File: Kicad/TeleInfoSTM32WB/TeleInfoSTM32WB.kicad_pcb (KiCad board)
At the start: 2 copper layers, 30 x 48.6 mm, 34 parts, among them J1 Conn_01x02_Female, J2 Conn_01x05_Female, J3 RSP-122811-01, J4 Conn_01x05_Female, SW1 SW_Push, U1 STM32WB55CCUx, U2 SFH620A-1, U3 LM2937xMP, Y1 32.768 KHz, Y2 Crystal_GND24

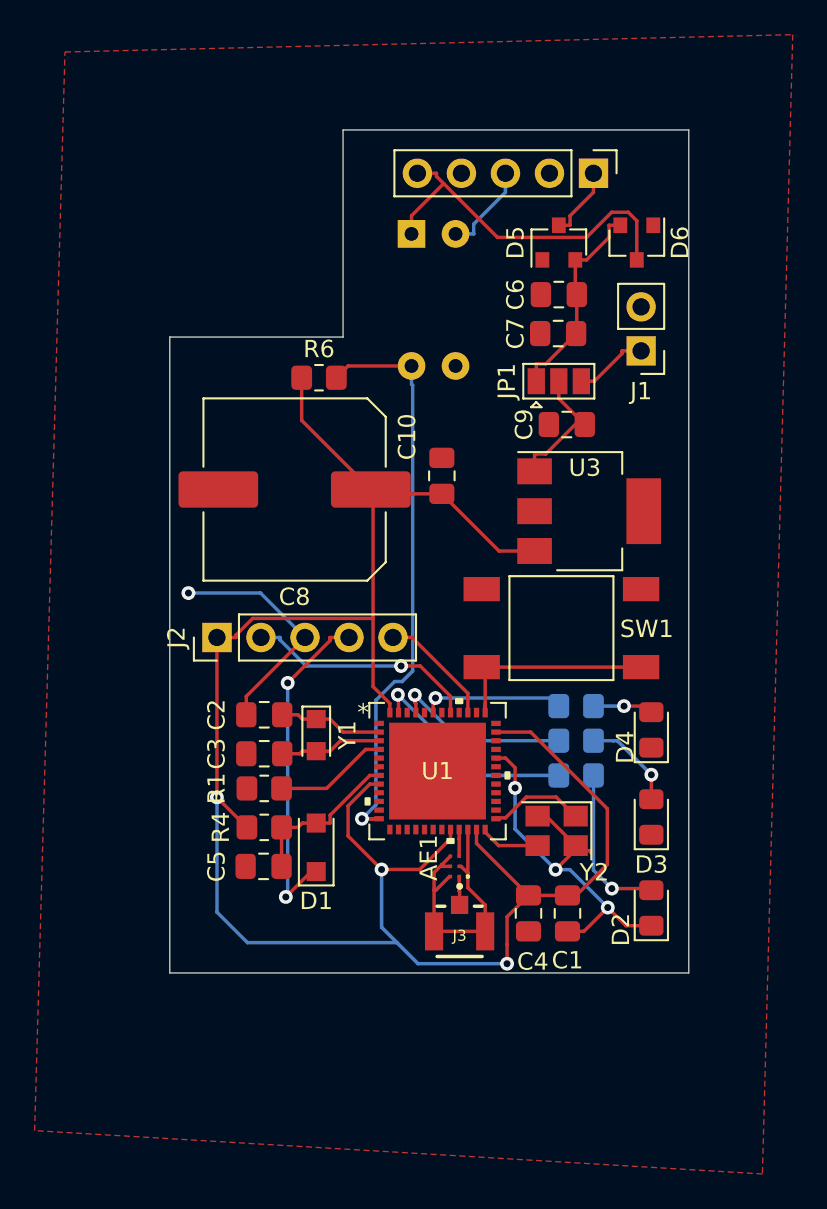
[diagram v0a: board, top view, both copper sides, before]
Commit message: PCB V6 (forget commited filed.... :clap:)
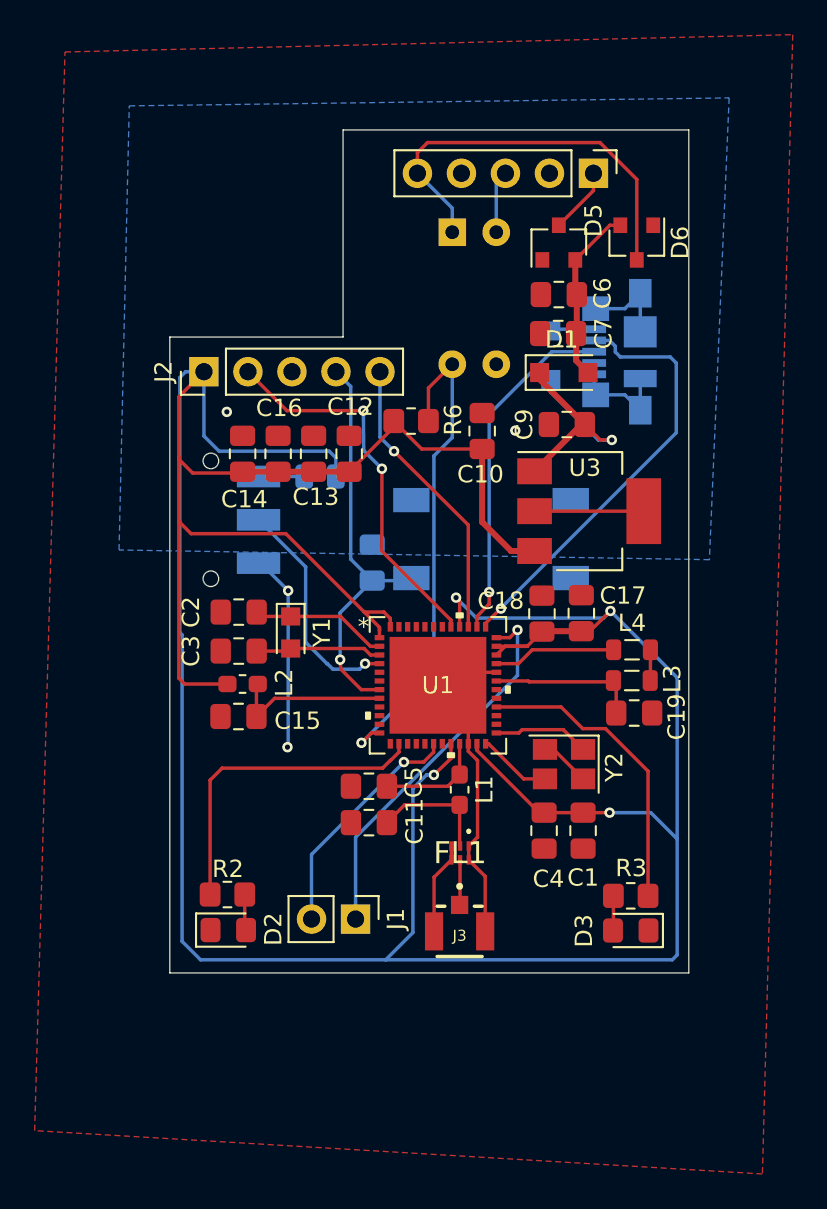
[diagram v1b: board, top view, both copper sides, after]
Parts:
- removed AE1: MLPF-WB55-01E3, MLPF-WB55-01E3:MLPF-WB55-01E3
- removed C8: 470mF, Capacitor_SMD:C_Elec_10x10.2
- removed JP1: Jumper_3_Open, Jumper:SolderJumper-3_P1.3mm_Open_Pad1.0x1.5mm
- removed R1: 10K, Resistor_SMD:R_0805_2012Metric_Pad1.20x1.40mm_HandSolder
- removed R4: 100K, Resistor_SMD:R_0805_2012Metric_Pad1.20x1.40mm_HandSolder
- removed R5: R750, Resistor_SMD:R_0805_2012Metric_Pad1.20x1.40mm_HandSolder
- added 4.7K1: R, Resistor_SMD:R_0805_2012Metric, B.Cu at (103.6, 104.7)
- added C11: 0.3pF, Capacitor_SMD:C_0805_2012Metric_Pad1.18x1.45mm_HandSolder, F.Cu at (106.4, 124.7)
- added C12: 100nF, Capacitor_SMD:C_0805_2012Metric_Pad1.18x1.45mm_HandSolder, F.Cu at (105.3, 103.4)
- added C13: 100nF, Capacitor_SMD:C_0805_2012Metric_Pad1.18x1.45mm_HandSolder, F.Cu at (103.2, 103.4)
- added C14: 100nF, Capacitor_SMD:C_0805_2012Metric_Pad1.18x1.45mm_HandSolder, F.Cu at (99.2, 103.4)
- added C15: 100nF, Capacitor_SMD:C_0805_2012Metric_Pad1.18x1.45mm_HandSolder, F.Cu at (98.9, 118.5)
- added C16: 100nF, Capacitor_SMD:C_0805_2012Metric_Pad1.18x1.45mm_HandSolder, F.Cu at (101.2, 103.4)
- added C17: 4.7uF, Capacitor_SMD:C_0805_2012Metric_Pad1.18x1.45mm_HandSolder, F.Cu at (118.7, 112.6)
- added C18: 100nF, Capacitor_SMD:C_0805_2012Metric_Pad1.18x1.45mm_HandSolder, F.Cu at (116.4, 112.6)
- added C19: 4.7uF, Capacitor_SMD:C_0805_2012Metric_Pad1.18x1.45mm_HandSolder, F.Cu at (121.8, 118.3)
- added C20: 100nF, Capacitor_SMD:C_0805_2012Metric_Pad1.18x1.45mm_HandSolder, B.Cu at (106.6, 109.7)
- added FL1: 2450LP14B100T, Customs:2450LP14B100T, F.Cu at (111.7, 126.4)
- added J5: USB_B_Micro, Connector_USB:USB_Micro-B_Molex_47346-0001, B.Cu at (120.9, 97.5)
- added L1: 2.7nH, Inductor_SMD:L_0603_1608Metric_Pad1.05x0.95mm_HandSolder, F.Cu at (111.7, 122.8)
- added L2: Z0603C601ASMST, Inductor_SMD:L_0603_1608Metric_Pad1.05x0.95mm_HandSolder, F.Cu at (99.2, 116.7)
- added L3: 10nH, Inductor_SMD:L_0805_2012Metric, F.Cu at (121.6, 116.5)
- added L4: 10nH, Inductor_SMD:L_0805_2012Metric, F.Cu at (121.6, 114.7)
- added SW2: SW_SPDT, Button_Switch_SMD:SW_SPDT_CK-JS102011SAQN, B.Cu at (97.3, 107.2)
- C5: value 100nF -> 0.8pF
- D1: value BAT54H -> D
- D4: value LED -> D; footprint LED_SMD:LED_0805_2012Metric_Pad1.15x1.40mm_HandSolder -> Diode_SMD:D_SOD-123F; moved to B.Cu
- J1: value Conn_01x02_Female -> Conn_01x02_Male
- R2, R3: moved to F.Cu
- SW1: moved to B.Cu
- U3: value LM2937xMP -> LM2937-IMP
- moved J1 36.7 mm to (105.7, 130.2), turned to 270 degrees
- moved D1 30.9 mm to (117.7, 98.7), turned to 0 degrees
- moved D2 24.4 mm to (98.3, 130.9), turned to 0 degrees
- moved D4 22.4 mm to (116.9, 97.7)
- moved R2 21.3 mm to (98.3, 128.8)
- moved J2 15.4 mm to (96.9, 98.7)
- moved R3 9.49 mm to (121.5, 128.9), turned to 0 degrees
- moved C5 7.64 mm to (106.4, 122.6), turned to 180 degrees
- moved D3 6.66 mm to (121.5, 130.9), turned to 180 degrees
- moved C2 6.11 mm to (98.9, 112.5)
- moved C3 6.11 mm to (98.9, 114.8)
- moved Y1 6.11 mm to (101.9, 113.7)
- moved R6 5.87 mm to (108.9, 101.5)
- moved SW1 5.13 mm to (123.0, 109.3), turned to 90 degrees
- moved U1 4.95 mm to (110.4, 116.8)
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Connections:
- C1 pad 1: +3V3 -> VBAT
- C10 pad 2: +3V3 -> VBAT
- C4 pad 1: +3V3 -> VBAT
- C5 pad 1: GND -> Net-(C5-Pad1)
- C5 pad 2: Net-(C5-Pad2) -> GND
- D1 pad 1: NRST -> Net-(C9-Pad2)
- D1 pad 2: Net-(C5-Pad2) -> Net-(C6-Pad1)
- D4 pad 1: GND -> Net-(C9-Pad2)
- D4 pad 2: Net-(D4-Pad2) -> +5V
- J1 pad 1: +5V -> BT_UART_RX
- J1 pad 2: GND -> BT_UART_TX
- J2 pad 1: +3V3 -> VBAT
- R6 pad 1: +3V3 -> VBAT
- SW1 pad 1: GND -> NRST
- SW1 pad 2: Net-(SW1-Pad2) -> GND
- U1 pad 1: Net-(U1-Pad1) -> VBAT
- U1 pad 14: Net-(U1-Pad14) -> Net-(R2-Pad2)
- U1 pad 18: Net-(U1-Pad18) -> BT_UART_TX
- U1 pad 20: +3V3 -> VBAT
- U1 pad 21: Net-(AE1-Pad3) -> Net-(C5-Pad1)
- U1 pad 23: +3V3 -> VBAT
- U1 pad 28: Net-(U1-Pad28) -> Net-(R3-Pad2)
- U1 pad 31: Net-(U1-Pad31) -> VFBFMPS
- U1 pad 33: Net-(U1-Pad33) -> VLXSMPS
- U1 pad 34: Net-(U1-Pad34) -> VBAT
- U1 pad 35: +3V3 -> VBAT
- U1 pad 36: Net-(U1-Pad36) -> BT_UART_RX
- U1 pad 37: Net-(SW1-Pad2) -> USB_DM
- U1 pad 38: Net-(U1-Pad38) -> USB_DP
- U1 pad 40: Net-(U1-Pad40) -> VBAT
- U1 pad 45: Net-(R3-Pad2) -> Net-(U1-Pad45)
- U1 pad 47: Net-(R2-Pad2) -> Net-(U1-Pad47)
- U1 pad 48: +3V3 -> VBAT
- U1 pad 49: Net-(U1-Pad49) -> GND
- U1 pad 7: Net-(C5-Pad2) -> NRST
- U1 pad 8: +3V3 -> VDDA
- U3 pad 3: +3V3 -> VBAT
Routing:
- net VBAT: track 0.00 -> 213.0 mm, vias 0 -> 4
- net +3V3: track 120.8 -> 0.00 mm, vias 3 -> 0
- net USB_DM: track 0.00 -> 25.3 mm, vias 0 -> 1
- net BT_UART_RX: track 0.00 -> 22.0 mm, vias 0 -> 1
- net USB_DP: track 0.00 -> 20.1 mm, vias 0 -> 1
- net BT_UART_TX: track 0.00 -> 13.8 mm, vias 0 -> 1
- net Net-(SW1-Pad2): track 13.7 -> 0.00 mm
- net SWDIO: track 6.77 -> 16.9 mm, vias 0 -> 1
- net VDDA: track 0.00 -> 9.44 mm
- net Net-(C5-Pad2): track 9.38 -> 0.00 mm
- net SWCLK: track 13.4 -> 22.2 mm, vias 1 -> 2
- net VFBFMPS: track 0.00 -> 8.74 mm
- net Net-(U1-Pad43): track 8.21 -> 0.00 mm, vias 1 -> 0
- net Net-(C9-Pad2): track 7.56 -> 15.5 mm, vias 0 -> 1
- net Net-(D2-Pad2): track 9.63 -> 2.08 mm, vias 1 -> 0
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- added copper zone on B.Cu, net GND
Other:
- board text added: "TeleInfo V6 - MHI 24/08/2021 STM32WB55CC"
- board text removed: "TeleInfo V4 - MHI 05/08/2021 STM32WB55CCUx"
